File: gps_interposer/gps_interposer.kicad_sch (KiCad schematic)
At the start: 9 parts, among them J1 Module Connector, J2 Carrier Connector, J3 Conn_01x10, U1 SN74LVC1T45DBV, U2 SN74LVC1T45DBV

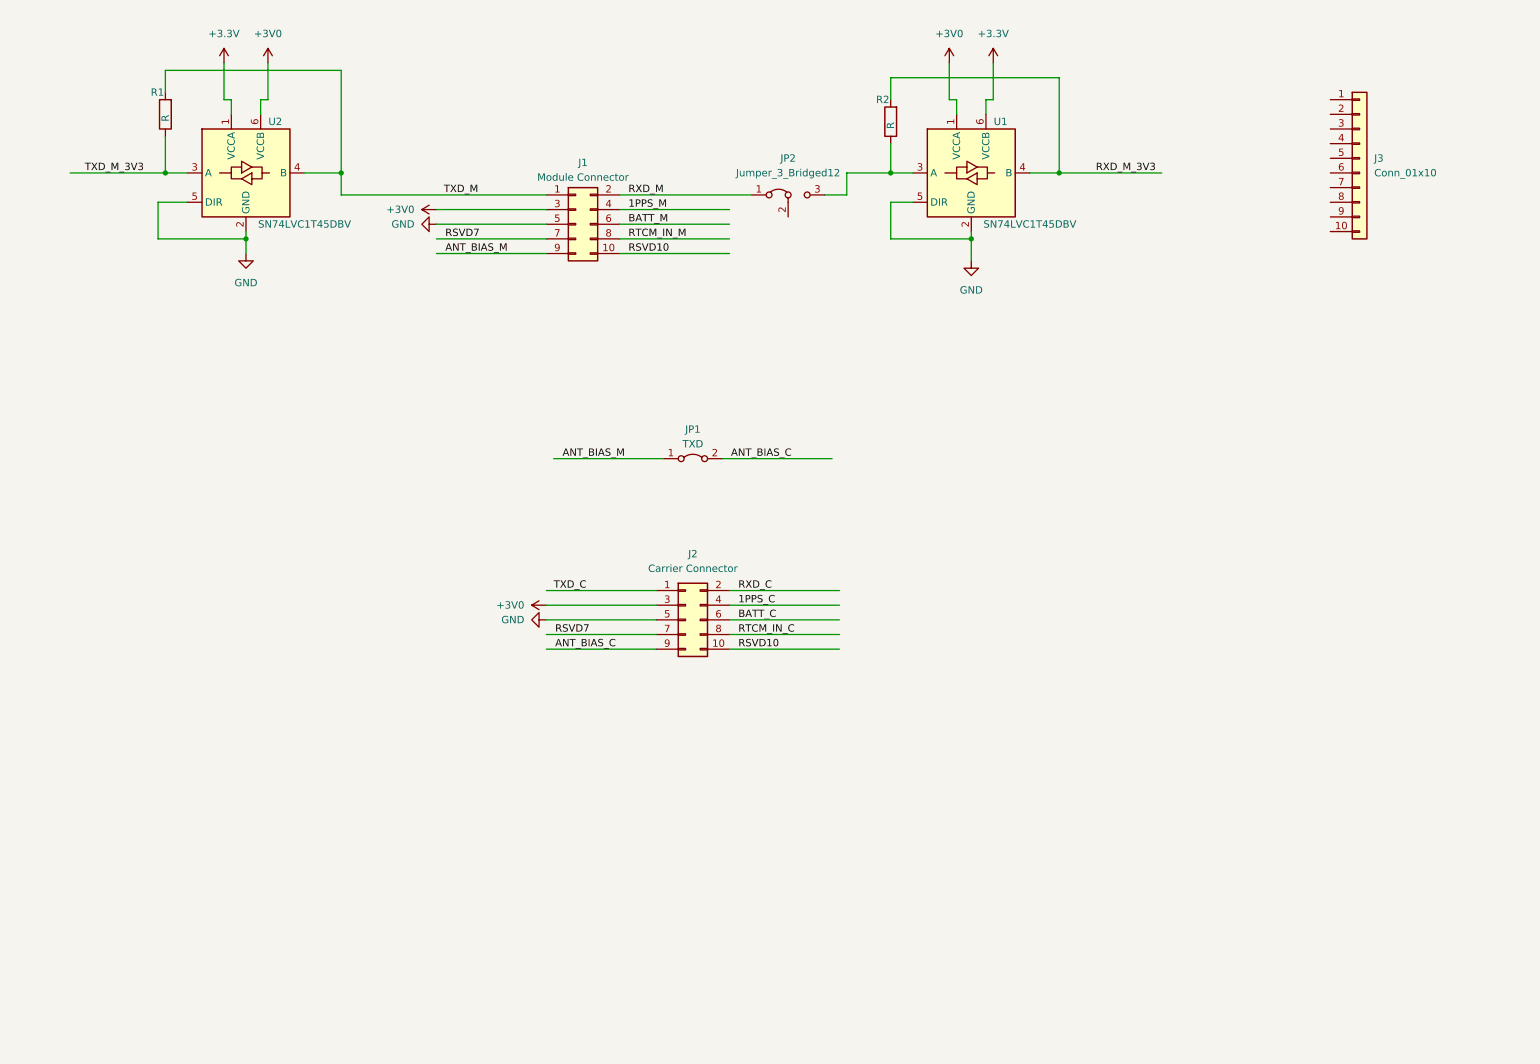
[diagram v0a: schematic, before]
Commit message: PCB almost done.
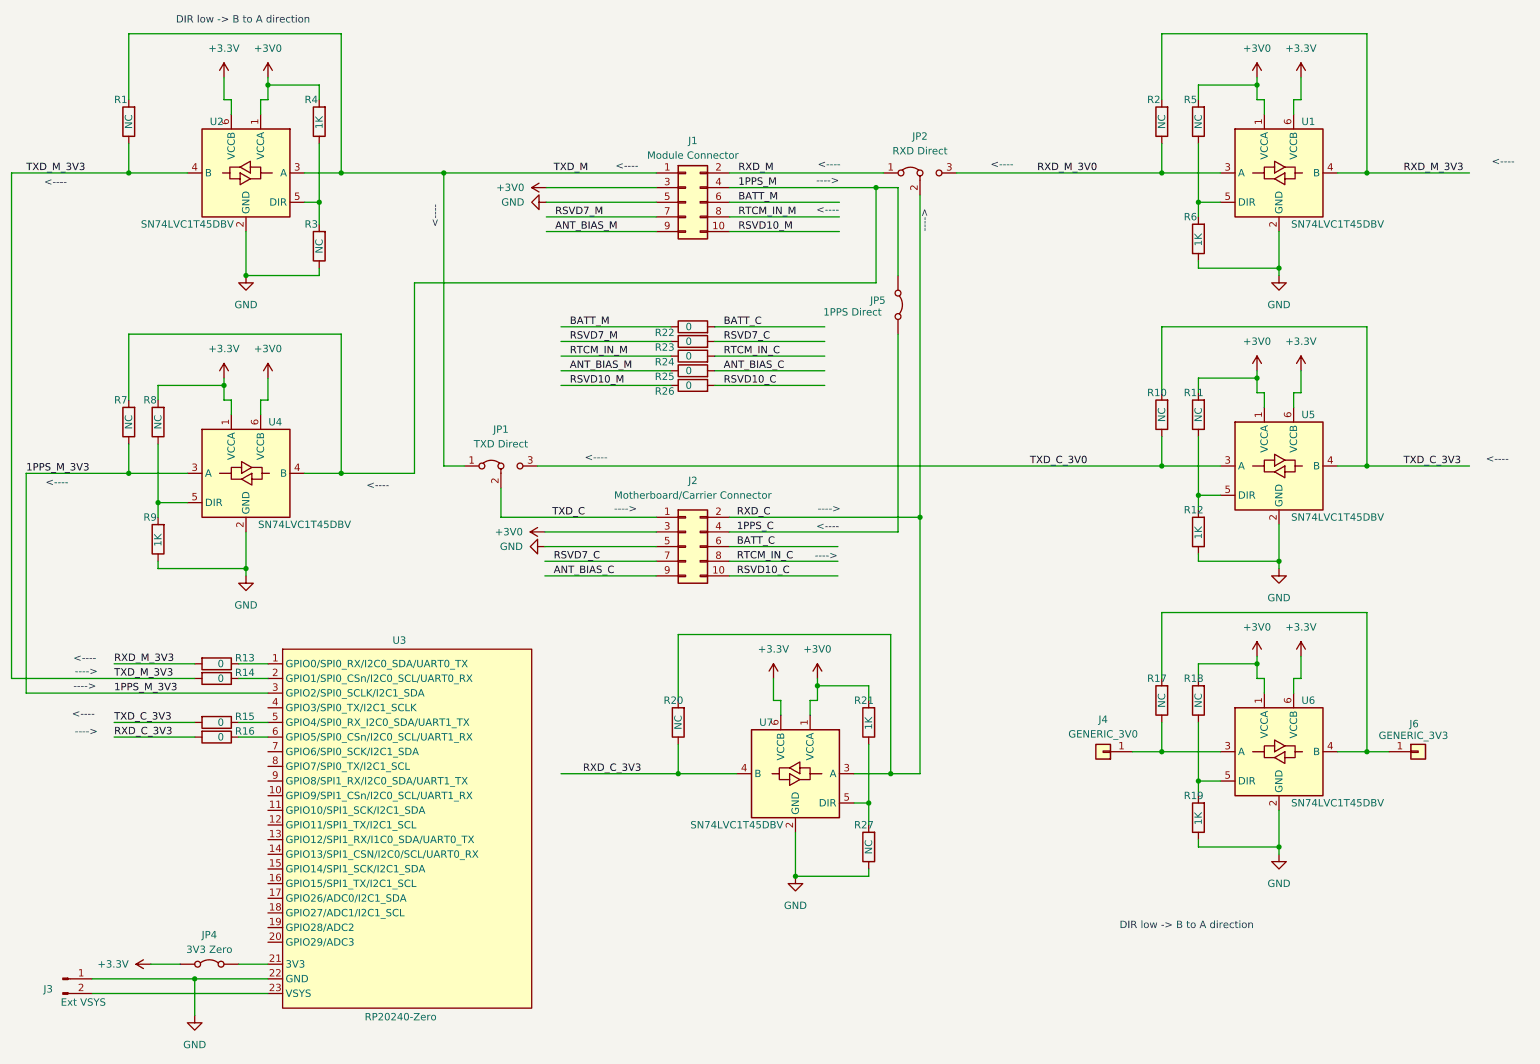
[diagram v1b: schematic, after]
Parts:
- removed J3: Conn_01x10, symbol Connector_Generic:Conn_01x10
- removed JP1: TXD, symbol Jumper:Jumper_2_Bridged
- added J3: Ext VSYS, Connector_PinHeader_2.54mm:PinHeader_1x02_P2.54mm_Horizontal, symbol Connector:Conn_01x02_Pin
- added J4: GENERIC_3V0, Connector_PinHeader_2.54mm:PinHeader_1x01_P2.54mm_Horizontal, symbol Connector_Generic:Conn_01x01
- added J6: GENERIC_3V3, Connector_PinHeader_2.54mm:PinHeader_1x01_P2.54mm_Horizontal, symbol Connector_Generic:Conn_01x01
- added JP1: TXD Direct, Connector_PinHeader_2.54mm:PinHeader_1x03_P2.54mm_Horizontal, symbol Jumper:Jumper_3_Bridged12
- added JP4: 3V3 Zero, Connector_PinHeader_2.54mm:PinHeader_1x02_P2.54mm_Horizontal, symbol Jumper:Jumper_2_Bridged
- added JP5: 1PPS Direct, Connector_PinHeader_2.54mm:PinHeader_1x02_P2.54mm_Horizontal, symbol Jumper:Jumper_2_Bridged
- added R10, R11, R17, R18, R20, R27, R3, R5, R7, R8: NC, Resistor_SMD:R_0603_1608Metric_Pad0.98x0.95mm_HandSolder, symbol Device:R
- added R12, R19, R21, R4, R6, R9: 1K, Resistor_SMD:R_0603_1608Metric_Pad0.98x0.95mm_HandSolder, symbol Device:R
- added R13, R14, R15, R16, R22, R23, R24, R25, R26: 0, Resistor_SMD:R_0603_1608Metric_Pad0.98x0.95mm_HandSolder, symbol Device:R
- added U3: RP20240-Zero, Kicad_Personal:RP2040-Zero, symbol Kicad_Personal:rp2040-zero
- added U4, U5, U6, U7: SN74LVC1T45DBV, Package_TO_SOT_SMD:SOT-23-6, symbol Logic_LevelTranslator:SN74LVC1T45DBV
- J1: footprint (none) -> Connector_PinSocket_1.27mm:PinSocket_2x05_P1.27mm_Vertical_SMD
- J2: value Carrier Connector -> Motherboard/Carrier Connector; footprint (none) -> Connector_PinHeader_1.27mm:PinHeader_2x05_P1.27mm_Vertical_SMD
- JP2: value Jumper_3_Bridged12 -> RXD Direct; footprint (none) -> Connector_PinHeader_2.54mm:PinHeader_1x03_P2.54mm_Horizontal
- R1, R2: value R -> NC; footprint (none) -> Resistor_SMD:R_0603_1608Metric_Pad0.98x0.95mm_HandSolder
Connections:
- net +3.3V: now also U2.6 (VCCB), JP4.1 (A), R8.2, U4.1 (VCCA), U5.6 (VCCB), U6.6 (VCCB), U7.6 (VCCB); no longer U2.1 (VCCA)
- net +3V0: now also U2.1 (VCCA), R11.2, R18.2, R21.2, R4.2, R5.2, U4.6 (VCCB), U5.1 (VCCA), U6.1 (VCCA), U7.1 (VCCA); no longer U2.6 (VCCB)
- net 1PPS_C: now also JP5.2 (B)
- net 1PPS_M: now also JP5.1 (A), R7.2, U4.4 (B)
- net ANT_BIAS_C: now also R25.2
- net ANT_BIAS_M: now also R25.1
- net BATT_C: now also R22.2
- net BATT_M: now also R22.1
- net GND: now also J3.1 (Pin_1), R12.1, R19.1, R27.1, R3.1, R6.1, R9.1, U3.22 (GND), U4.2 (GND), U5.2 (GND), U6.2 (GND), U7.2 (GND); no longer U1.5 (DIR), U2.5 (DIR)
- net RTCM_IN_C: now also R24.2
- net RTCM_IN_M: now also R24.1
- net RXD_C: now also JP2.2 (C), R20.2, U7.3 (A)
- net RXD_M_3V3: now also R13.2
- net TXD_C: now also JP1.2 (C)
- net TXD_M: now also U2.3 (A), JP1.1 (A); no longer U2.4 (B)
- net TXD_M_3V3: now also U2.4 (B), R14.2; no longer U2.3 (A)
- net RXD_M_3V0: now reaches JP2.3 (B), R2.1, U1.3 (A)
- net RSVD10 renamed RSVD10_C
- net RSVD10_C: now also R26.2; no longer J1.10 (Pin_10)
- net RSVD7 renamed RSVD7_C
- net RSVD7_C: now also R23.2; no longer J1.7 (Pin_7)
- new net: J4.1 (Pin_1), R17.1, U6.3 (A)
- new net: J6.1 (Pin_1), R17.2, U6.4 (B)
- new net: R21.1, R27.2, U7.5 (DIR)
- new net: R8.1, R9.2, U4.5 (DIR)
- new net: R13.1, U3.1 (GPIO0/SPI0_RX/I2C0_SDA/UART0_TX)
- new net: R14.1, U3.2 (GPIO1/SPI0_CSn/I2C0_SCL/UART0_RX)
- new net: JP4.2 (B), U3.21 (3V3)
- new net: J3.2 (Pin_2), U3.23 (VSYS)
- new net: R15.1, U3.5 (GPIO4/SPI0_RX_I2C0_SDA/UART1_TX)
- new net: R16.1, U3.6 (GPIO5/SPI0_CSn/I2C0_SCL/UART1_RX)
- new net: R5.1, R6.2, U1.5 (DIR)
- new net: R11.1, R12.2, U5.5 (DIR)
- new net: R3.2, R4.1, U2.5 (DIR)
- new net: R18.1, R19.2, U6.5 (DIR)
- new net 1PPS_M_3V3: R7.1, U3.3 (GPIO2/SPI0_SCLK/I2C1_SDA), U4.3 (A)
- new net RSVD10_M: J1.10 (Pin_10), R26.1
- new net RSVD7_M: J1.7 (Pin_7), R23.1
- new net RXD_C_3V3: R16.2, R20.1, U7.4 (B)
- new net TXD_C_3V0: JP1.3 (B), R10.1, U5.3 (A)
- new net TXD_C_3V3: R10.2, R15.2, U5.4 (B)
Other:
- note added: "---->"
- note added: "<----"
- note added: "DIR low -> B to A direction"
- moved on the sheet: J1, J2, JP2, R1, R2, U1
